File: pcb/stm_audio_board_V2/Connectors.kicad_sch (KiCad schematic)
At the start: 12 parts, among them J1 Power conn, J2 STlink, J3 Audio_sig, J4 Conn_01x10_display TODO, J4 Conn_01x10_pots_internal, J5 SPI, J6 Conn_01x03_pot_ext, J6 Conn_01x03_taptempo

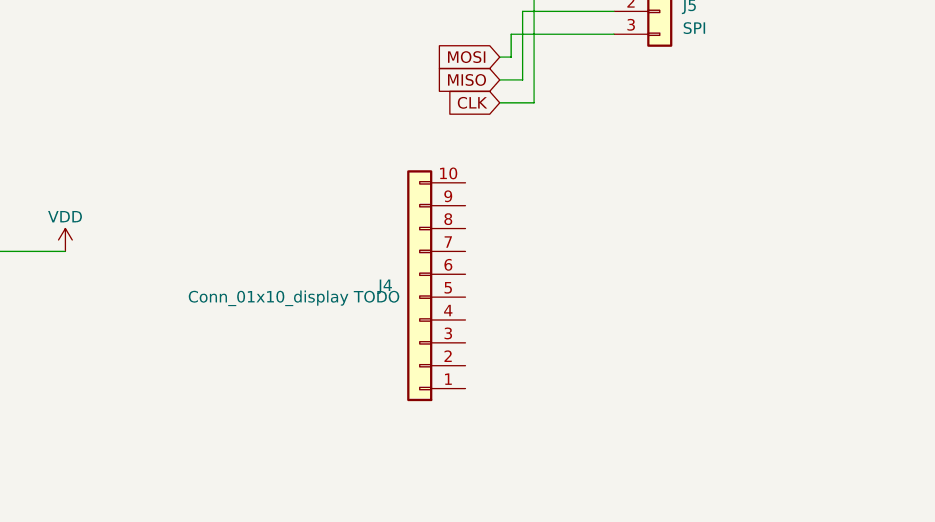
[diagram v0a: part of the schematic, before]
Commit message: pinsetup ready
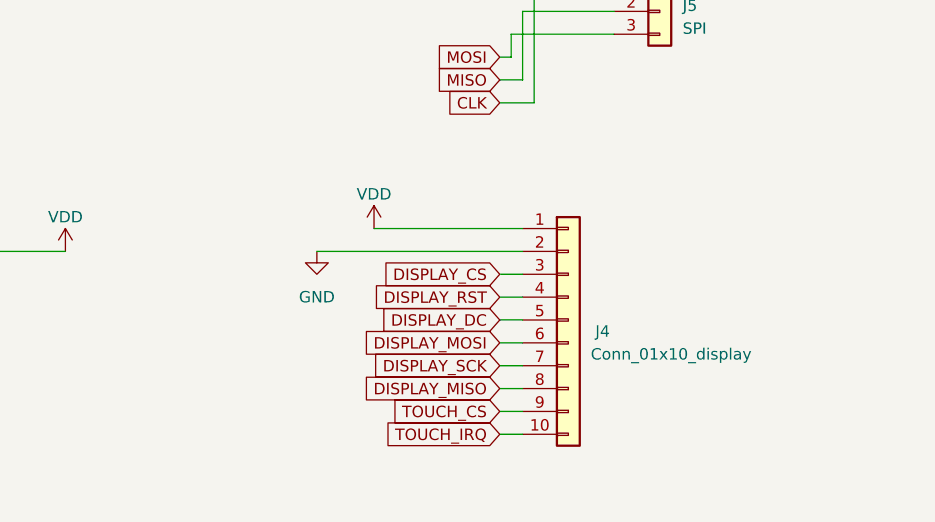
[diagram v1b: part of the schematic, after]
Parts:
- J4: value Conn_01x10_display TODO -> Conn_01x10_display
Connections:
- net GND: now also J4.2 (Pin_2)
- net VDD: now also J4.1 (Pin_1)
- net TOUCH_IRQ: now reaches J4.10 (Pin_10)
- net DISPLAY_CS: now reaches J4.3 (Pin_3)
- net DISPLAY_RST: now reaches J4.4 (Pin_4)
- net DISPLAY_DC: now reaches J4.5 (Pin_5)
- net DISPLAY_MOSI: now reaches J4.6 (Pin_6)
- net DISPLAY_SCK: now reaches J4.7 (Pin_7)
- net DISPLAY_MISO: now reaches J4.8 (Pin_8)
- net TOUCH_CS: now reaches J4.9 (Pin_9)
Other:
- moved on the sheet: J4
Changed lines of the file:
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@@
+    (stroke (width 0) (type default))
+  )
+  (wire (pts (xy 119.38 132.08) (xy 121.92 132.08))
     (stroke (width 0) (type default))
   )
@@
     (stroke (width 0) (type default))
   )
+  (wire (pts (xy 119.38 134.62) (xy 121.92 134.62))
+    (stroke (width 0) (type default))
+  )
   (wire (pts (xy 48.26 143.51) (xy 57.15 143.51))
     (stroke (width 0) (type default))
@@
     (stroke (width 0) (type default))
   )
+  (wire (pts (xy 119.38 127) (xy 121.92 127))
+    (stroke (width 0) (type default))
+  )
+  (wire (pts (xy 119.38 137.16) (xy 121.92 137.16))
+    (stroke (width 0) (type default))
+  )
   (wire (pts (xy 46.99 101.6) (xy 50.8 101.6))
     (stroke (width 0) (type default))
@@
     (stroke (width 0) (type default))
   )
+  (wire (pts (xy 119.38 139.7) (xy 121.92 139.7))
+    (stroke (width 0) (type default))
+  )
+  (wire (pts (xy 105.41 119.38) (xy 121.92 119.38))
+    (stroke (width 0) (type default))
+  )
+  (wire (pts (xy 119.38 124.46) (xy 121.92 124.46))
+    (stroke (width 0) (type default))
+  )
   (wire (pts (xy 146.05 40.64) (xy 142.24 40.64))
     (stroke (width 0) (type default))
@@
     (stroke (width 0) (type default))
   )
+  (wire (pts (xy 99.06 121.92) (xy 121.92 121.92))
+    (stroke (width 0) (type default))
+  )
   (wire (pts (xy 105.41 39.37) (xy 113.03 39.37))
     (stroke (width 0) (type default))
@@
     (stroke (width 0) (type default))
   )
+  (wire (pts (xy 119.38 142.24) (xy 121.92 142.24))
+    (stroke (width 0) (type default))
+  )
   (wire (pts (xy 142.24 35.56) (xy 146.05 35.56))
     (stroke (width 0) (type default))
@@
   )
   (wire (pts (xy 46.99 106.68) (xy 50.8 106.68))
+    (stroke (width 0) (type default))
+  )
+  (wire (pts (xy 119.38 129.54) (xy 121.92 129.54))
     (stroke (width 0) (type default))
   )
@@
     (effects (font (size 1.27 1.27)) (justify left bottom))
   )
+  (global_label "DISPLAY_DC" (shape input) (at 119.38 129.54 180) (fields_autoplaced)
+    (effects (font (size 1.27 1.27)) (justify right))
+    (property "Intersheetrefs" "${INTERSHEET_REFS}" (at 105.407 129.54 0)
+      (effects (font (size 1.27 1.27)) (justify right) hide)
+    )
+  )
   (global_label "POT3" (shape input) (at 50.8 106.68 0) (fields_autoplaced)
     (effects (font (size 1.27 1.27)) (justify left))
@@
     )
   )
+  (global_label "DISPLAY_RST" (shape input) (at 119.38 127 180) (fields_autoplaced)
+    (effects (font (size 1.27 1.27)) (justify right))
+    (property "Intersheetrefs" "${INTERSHEET_REFS}" (at 104.4999 127 0)
+      (effects (font (size 1.27 1.27)) (justify right) hide)
+    )
+  )
   (global_label "POT7" (shape input) (at 50.8 116.84 0) (fields_autoplaced)
     (effects (font (size 1.27 1.27)) (justify left))
@@
     )
   )
+  (global_label "TOUCH_CS" (shape input) (at 119.38 139.7 180) (fields_autoplaced)
+    (effects (font (size 1.27 1.27)) (justify right))
+    (property "Intersheetrefs" "${INTERSHEET_REFS}" (at 106.798 139.7 0)
+      (effects (font (size 1.27 1.27)) (justify right) hide)
+    )
+  )
   (global_label "TAP_TEMPO_INPUT" (shape input) (at 158.75 68.58 0) (fields_autoplaced)
     (effects (font (size 1.27 1.27)) (justify left))
@@
     )
   )
+  (global_label "DISPLAY_SCK" (shape input) (at 119.38 134.62 180) (fields_autoplaced)
+    (effects (font (size 1.27 1.27)) (justify right))
+    (property "Intersheetrefs" "${INTERSHEET_REFS}" (at 104.1975 134.62 0)
+      (effects (font (size 1.27 1.27)) (justify right) hide)
+    )
+  )
   (global_label "SWCLK" (shape input) (at 146.05 35.56 0) (fields_autoplaced)
     (effects (font (size 1.27 1.27)) (justify left))
@@
     )
   )
+  (global_label "DISPLAY_CS" (shape input) (at 119.38 124.46 180) (fields_autoplaced)
+    (effects (font (size 1.27 1.27)) (justify right))
+    (property "Intersheetrefs" "${INTERSHEET_REFS}" (at 105.4675 124.46 0)
+      (effects (font (size 1.27 1.27)) (justify right) hide)
+    )
+  )
   (global_label "POT8" (shape input) (at 50.8 119.38 0) (fields_autoplaced)
     (effects (font (size 1.27 1.27)) (justify left))
@@
     )
   )
+  (global_label "TOUCH_IRQ" (shape input) (at 119.38 142.24 180) (fields_autoplaced)
+    (effects (font (size 1.27 1.27)) (justify right))
+    (property "Intersheetrefs" "${INTERSHEET_REFS}" (at 106.0722 142.24 0)
+      (effects (font (size 1.27 1.27)) (justify right) hide)
+    )
+  )
   (global_label "MOSI" (shape input) (at 119.38 100.33 180) (fields_autoplaced)
     (effects (font (size 1.27 1.27)) (justify right))
@@
     )
   )
+  (global_label "DISPLAY_MOSI" (shape input) (at 119.38 132.08 180) (fields_autoplaced)
+    (effects (font (size 1.27 1.27)) (justify right))
+    (property "Intersheetrefs" "${INTERSHEET_REFS}" (at 103.3508 132.08 0)
+      (effects (font (size 1.27 1.27)) (justify right) hide)
+    )
+  )
   (global_label "POT2" (shape input) (at 50.8 104.14 0) (fields_autoplaced)
     (effects (font (size 1.27 1.27)) (justify left))
@@
     (property "Intersheetrefs" "${INTERSHEET_REFS}" (at 76.2634 81.28 0)
       (effects (font (size 1.27 1.27)) (justify left) hide)
+    )
+  )
+  (global_label "DISPLAY_MISO" (shape input) (at 119.38 137.16 180) (fields_autoplaced)
+    (effects (font (size 1.27 1.27)) (justify right))
+    (property "Intersheetrefs" "${INTERSHEET_REFS}" (at 103.3508 137.16 0)
+      (effects (font (size 1.27 1.27)) (justify right) hide)
     )
   )
@@
     )
   )
+  (symbol (lib_id "power:GND") (at 99.06 121.92 0) (unit 1)
+    (in_bom yes) (on_board yes) (dnp no) (fields_autoplaced)
+    (property "Reference" "#PWR052" (at 99.06 128.27 0)
+      (effects (font (size 1.27 1.27)) hide)
+    )
+    (property "Value" "GND" (at 99.06 127 0)
+      (effects (font (size 1.27 1.27)))
+    )
+    (property "Footprint" "" (at 99.06 121.92 0)
+      (effects (font (size 1.27 1.27)) hide)
+    )
+    (property "Datasheet" "" (at 99.06 121.92 0)
+      (effects (font (size 1.27 1.27)) hide)
+    )
+    (pin "1")
+    (instances
+      (project "stm_audio_board_V2"
+        (path "/6997cf63-2615-4e49-9471-e7da1b6bae71"
+          (reference "#PWR052") (unit 1)
+        )
+        (path "/6997cf63-2615-4e49-9471-e7da1b6bae71/6424856c-1346-4018-a943-0d16008c9545"
+          (reference "#PWR095") (unit 1)
+        )
+      )
+    )
+  )
   (symbol (lib_id "power:GND") (at 146.05 41.91 0) (unit 1)
     (in_bom yes) (on_board yes) (dnp no) (fields_autoplaced)
@@
     )
   )
-  (symbol (lib_id "Connector_Generic:Conn_01x10") (at 110.49 127 180) (unit 1)
+  (symbol (lib_id "Connector_Generic:Conn_01x10") (at 127 129.54 0) (unit 1)
     (in_bom yes) (on_board yes) (dnp no)
-    (property "Reference" "J4" (at 106.68 125.73 0)
-      (effects (font (size 1.27 1.27)))
-    )
-    (property "Value" "Conn_01x10_display TODO" (at 96.52 127 0)
-      (effects (font (size 1.27 1.27)))
-    )
-    (property "Footprint" "Connector_PinHeader_2.54mm:PinHeader_1x10_P2.54mm_Vertical" (at 110.49 127 0)
-      (effects (font (size 1.27 1.27)) hide)
-    )
-    (property "Datasheet" "~" (at 110.49 127 0)
+    (property "Reference" "J4" (at 130.81 130.81 0)
+      (effects (font (size 1.27 1.27)))
+    )
+    (property "Value" "Conn_01x10_display" (at 138.43 133.35 0)
+      (effects (font (size 1.27 1.27)))
+    )
+    (property "Footprint" "Connector_PinHeader_2.54mm:PinHeader_1x10_P2.54mm_Vertical" (at 127 129.54 0)
+      (effects (font (size 1.27 1.27)) hide)
+    )
+    (property "Datasheet" "~" (at 127 129.54 0)
       (effects (font (size 1.27 1.27)) hide)
     )
@@
         )
       )
+    )
+  )
+  (symbol (lib_id "power:VDD") (at 105.41 119.38 0) (unit 1)
+    (in_bom yes) (on_board yes) (dnp no) (fields_autoplaced)
+    (property "Reference" "#PWR051" (at 105.41 123.19 0)
+      (effects (font (size 1.27 1.27)) hide)
+    )
+    (property "Value" "VDD" (at 105.41 115.57 0)
+      (effects (font (size 1.27 1.27)))
+    )
+    (property "Footprint" "" (at 105.41 119.38 0)
+      (effects (font (size 1.27 1.27)) hide)
+    )
+    (property "Datasheet" "" (at 105.41 119.38 0)
+      (effects (font (size 1.27 1.27)) hide)
+    )
+    (pin "1")
+    (instances
+      (project "stm_audio_board_V2"
+        (path "/6997cf63-2615-4e49-9471-e7da1b6bae71"
+          (reference "#PWR051") (unit 1)
+        )
+        (path "/6997cf63-2615-4e49-9471-e7da1b6bae71/6424856c-1346-4018-a943-0d16008c9545"
+          (reference "#PWR036") (unit 1)
+        )
+      )
